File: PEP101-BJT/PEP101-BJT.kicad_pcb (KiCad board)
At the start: 2 copper layers, 45 x 45 mm, 15 parts, among them J1 Screw_Terminal_01x02, J3 Conn_01x02_Pin, J4 Conn_01x02_Pin, J5 Conn_01x02_Pin, J6 Conn_01x02_Pin, Q2 MMBT5551L

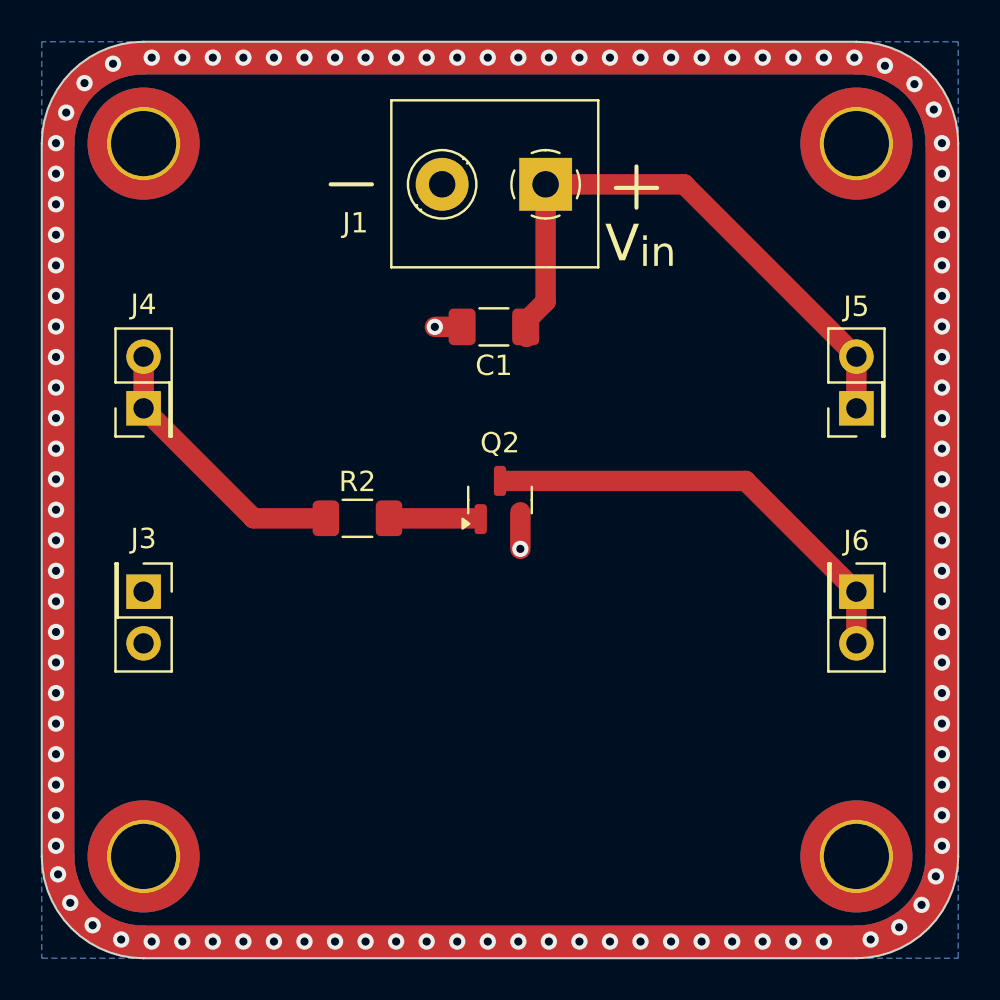
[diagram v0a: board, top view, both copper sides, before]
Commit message: fix
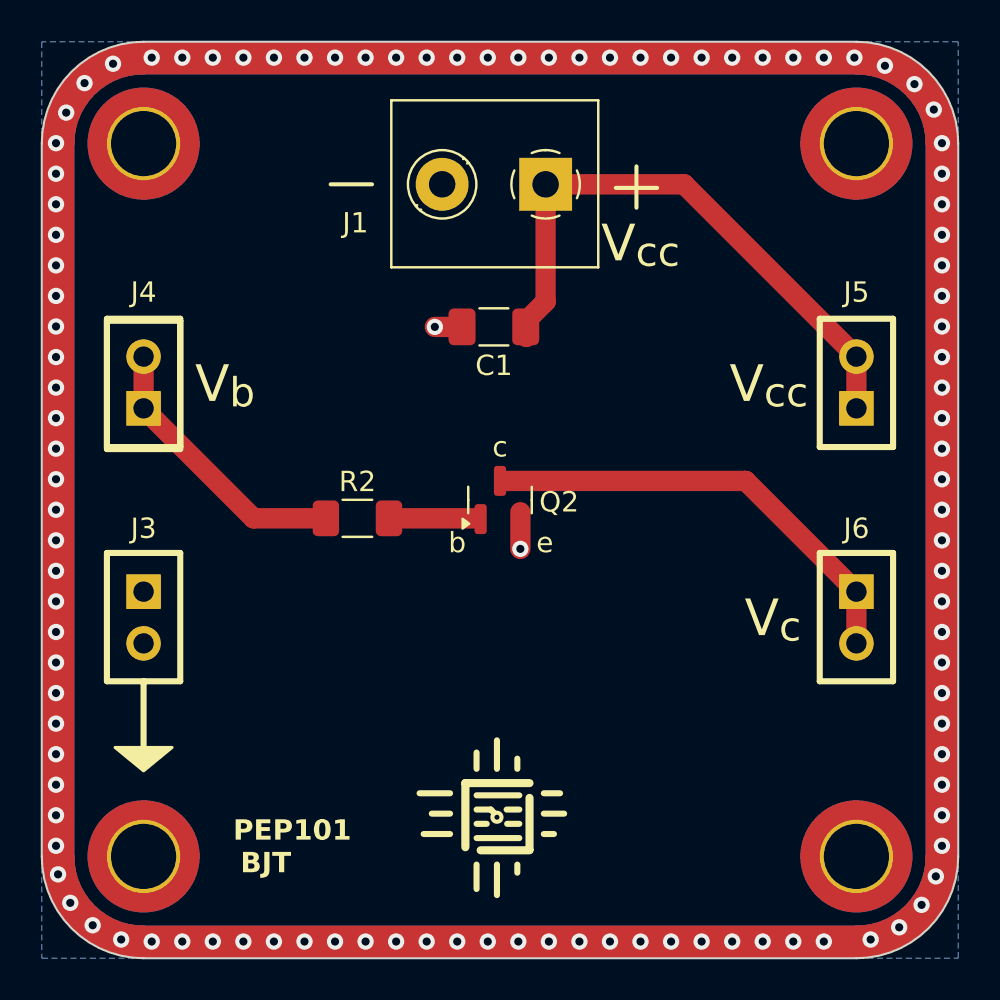
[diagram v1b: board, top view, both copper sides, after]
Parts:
- added REF**: ele_petnica_logo, PEP_library:ele_petnica_logo, F.Cu at (122.3, 138.1)
- J3, J4, J5, J6: footprint Connector_PinHeader_2.54mm:PinHeader_2x01_P2.54mm_Vertical -> PEP_library:PinHeader_2x01_P2.54mm_Vertical
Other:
- board text added: "BJT"
- board text added: "PEP101"
- board text added: "V_{b}"
- board text added: "V_{cc}"
- board text added: "V_{c}"
- board text added: "b"
- board text added: "c"
- board text added: "e"
